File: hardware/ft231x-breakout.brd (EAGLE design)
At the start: 26.7 x 15.2 mm, 27 parts, among them Q1 2N7002PW, U1 FT231XS

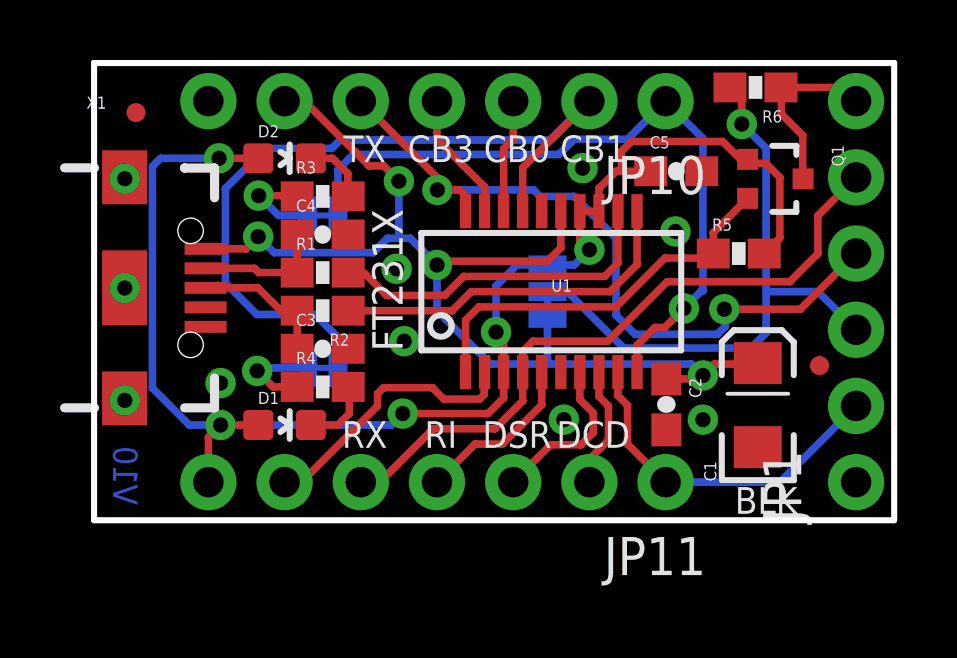
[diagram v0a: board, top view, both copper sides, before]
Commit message: Silk Change
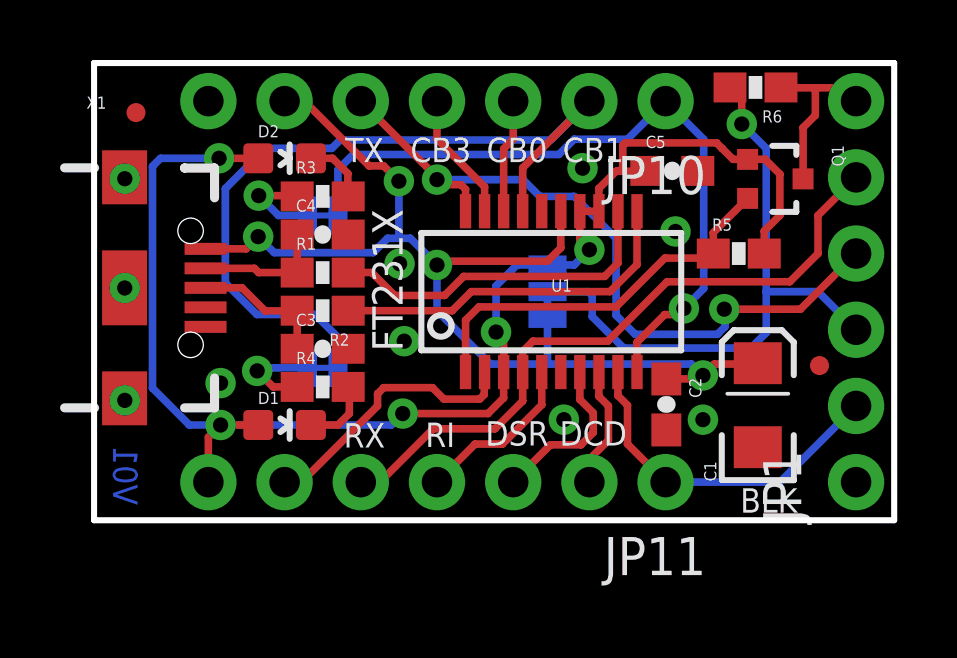
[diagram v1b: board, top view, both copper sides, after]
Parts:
- moved FRAME1 4.02 mm to (-11.4, -11.4)
- moved C5 0.13 mm to (19.3, 11.6)
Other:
- board text added: "V01"
- board text removed: "V10"
